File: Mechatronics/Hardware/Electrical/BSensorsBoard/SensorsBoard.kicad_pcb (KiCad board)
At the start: 2 copper layers, 49.8 x 13.7 mm, 10 parts, among them J1 Conn_01x01_Male, J2 Conn_01x01_Male, J3 Conn_01x01_Male, J4 Conn_01x01_Male, J5 Conn_01x01_Male, J6 Conn_01x01_Male, J7 Conn_01x01_Male, J8 Conn_01x01_Male, U1 ITR1802, U2 ITR1802

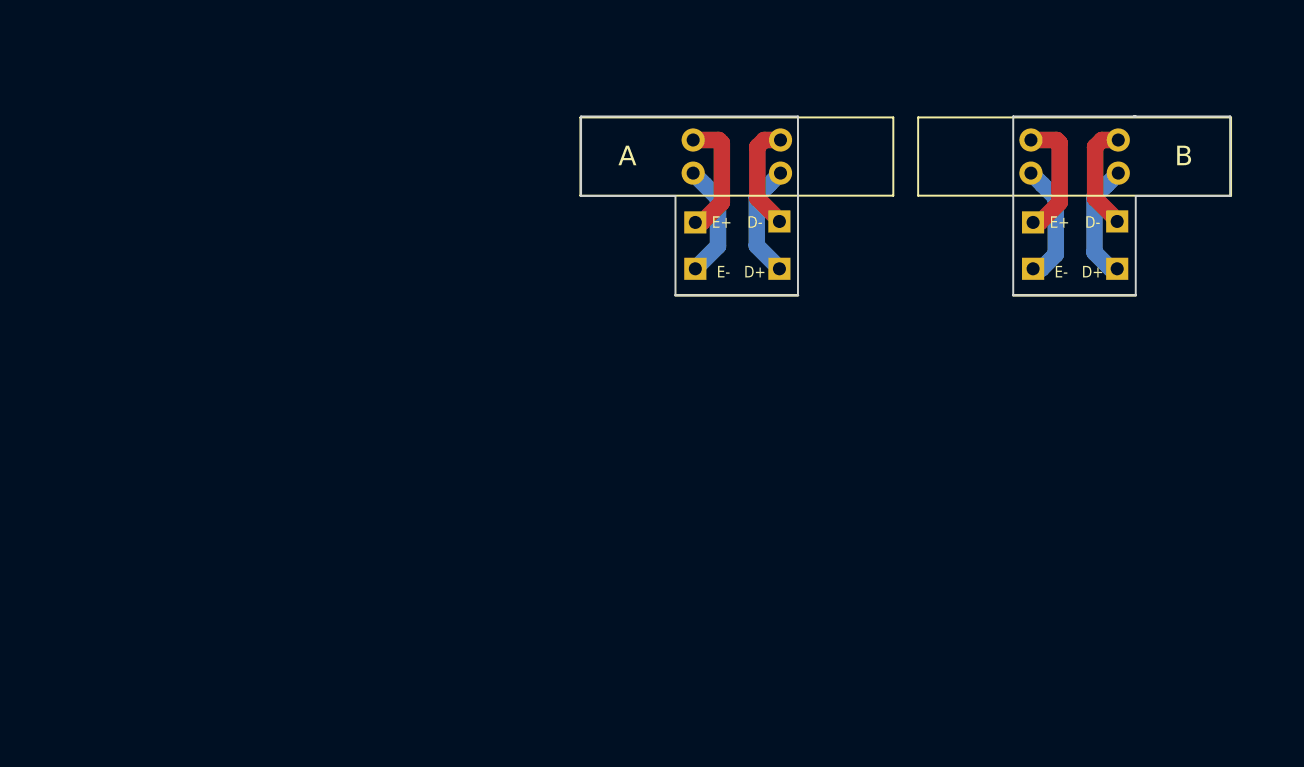
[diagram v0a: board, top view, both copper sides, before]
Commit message: Added changes
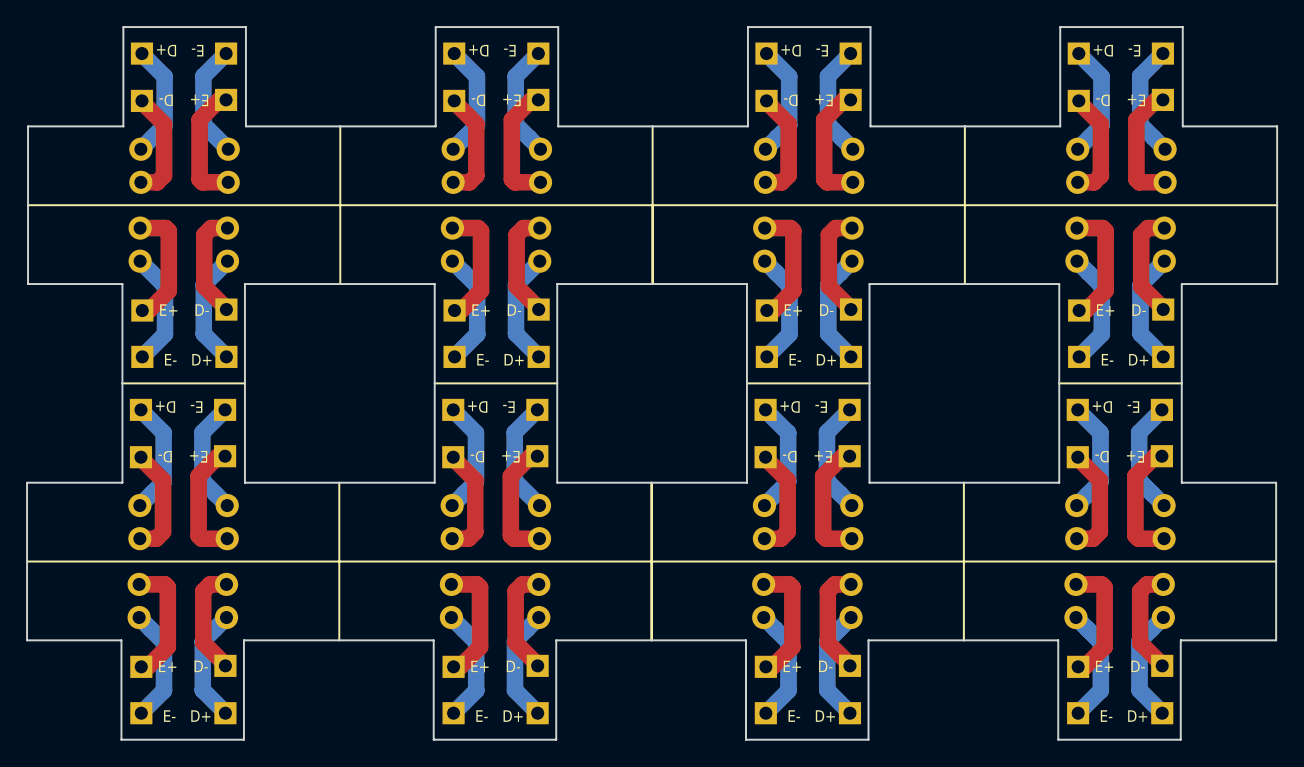
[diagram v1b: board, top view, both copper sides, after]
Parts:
- removed J5, J6, J7, J8: Conn_01x01_Male, Encoder:No3dmodelPinHeader_1x01_P2.54mm_Vertical
- removed U2: ITR1802, Encoder:itr8102
- added J1: Conn_01x01_Male, Encoder:No3dmodelPinHeader_1x01_P2.54mm_Vertical, F.Cu at (150.7, 120.2)
- added J1: Conn_01x01_Male, Encoder:No3dmodelPinHeader_1x01_P2.54mm_Vertical, F.Cu at (109.3, 76.7)
- added J1: Conn_01x01_Male, Encoder:No3dmodelPinHeader_1x01_P2.54mm_Vertical, F.Cu at (126.8, 92.9)
- added J1: Conn_01x01_Male, Encoder:No3dmodelPinHeader_1x01_P2.54mm_Vertical, F.Cu at (102.9, 92.9)
- added J1: Conn_01x01_Male, Encoder:No3dmodelPinHeader_1x01_P2.54mm_Vertical, F.Cu at (109.2, 104.0)
- added J1: Conn_01x01_Male, Encoder:No3dmodelPinHeader_1x01_P2.54mm_Vertical, F.Cu at (133.2, 104.0)
- added J1: Conn_01x01_Male, Encoder:No3dmodelPinHeader_1x01_P2.54mm_Vertical, F.Cu at (126.7, 120.2)
- added J1: Conn_01x01_Male, Encoder:No3dmodelPinHeader_1x01_P2.54mm_Vertical, F.Cu at (174.7, 120.2)
- added J1: Conn_01x01_Male, Encoder:No3dmodelPinHeader_1x01_P2.54mm_Vertical, F.Cu at (157.1, 104.0)
- added J1: Conn_01x01_Male, Encoder:No3dmodelPinHeader_1x01_P2.54mm_Vertical, F.Cu at (181.1, 104.0)
- added J1: Conn_01x01_Male, Encoder:No3dmodelPinHeader_1x01_P2.54mm_Vertical, F.Cu at (150.8, 92.9)
- added J1: Conn_01x01_Male, Encoder:No3dmodelPinHeader_1x01_P2.54mm_Vertical, F.Cu at (174.7, 92.9)
- added J1: Conn_01x01_Male, Encoder:No3dmodelPinHeader_1x01_P2.54mm_Vertical, F.Cu at (157.2, 76.7)
- added J1: Conn_01x01_Male, Encoder:No3dmodelPinHeader_1x01_P2.54mm_Vertical, F.Cu at (181.2, 76.7)
- added J1: Conn_01x01_Male, Encoder:No3dmodelPinHeader_1x01_P2.54mm_Vertical, F.Cu at (133.2, 76.7)
- added J2: Conn_01x01_Male, Encoder:No3dmodelPinHeader_1x01_P2.54mm_Vertical, F.Cu at (150.8, 96.4)
- added J2: Conn_01x01_Male, Encoder:No3dmodelPinHeader_1x01_P2.54mm_Vertical, F.Cu at (102.9, 96.4)
- added J2: Conn_01x01_Male, Encoder:No3dmodelPinHeader_1x01_P2.54mm_Vertical, F.Cu at (133.2, 73.2)
- added J2: Conn_01x01_Male, Encoder:No3dmodelPinHeader_1x01_P2.54mm_Vertical, F.Cu at (126.8, 96.4)
- added J2: Conn_01x01_Male, Encoder:No3dmodelPinHeader_1x01_P2.54mm_Vertical, F.Cu at (109.2, 100.5)
- added J2: Conn_01x01_Male, Encoder:No3dmodelPinHeader_1x01_P2.54mm_Vertical, F.Cu at (133.2, 100.5)
- added J2: Conn_01x01_Male, Encoder:No3dmodelPinHeader_1x01_P2.54mm_Vertical, F.Cu at (126.7, 123.7)
- added J2: Conn_01x01_Male, Encoder:No3dmodelPinHeader_1x01_P2.54mm_Vertical, F.Cu at (174.7, 123.7)
- added J2: Conn_01x01_Male, Encoder:No3dmodelPinHeader_1x01_P2.54mm_Vertical, F.Cu at (181.1, 100.5)
- added J2: Conn_01x01_Male, Encoder:No3dmodelPinHeader_1x01_P2.54mm_Vertical, F.Cu at (150.7, 123.7)
- added J2: Conn_01x01_Male, Encoder:No3dmodelPinHeader_1x01_P2.54mm_Vertical, F.Cu at (157.1, 100.5)
- added J2: Conn_01x01_Male, Encoder:No3dmodelPinHeader_1x01_P2.54mm_Vertical, F.Cu at (157.2, 73.2)
- added J2: Conn_01x01_Male, Encoder:No3dmodelPinHeader_1x01_P2.54mm_Vertical, F.Cu at (181.2, 73.2)
- added J2: Conn_01x01_Male, Encoder:No3dmodelPinHeader_1x01_P2.54mm_Vertical, F.Cu at (174.7, 96.4)
- added J2: Conn_01x01_Male, Encoder:No3dmodelPinHeader_1x01_P2.54mm_Vertical, F.Cu at (109.3, 73.2)
- added J3: Conn_01x01_Male, Encoder:No3dmodelPinHeader_1x01_P2.54mm_Vertical, F.Cu at (150.7, 76.8)
- added J3: Conn_01x01_Male, Encoder:No3dmodelPinHeader_1x01_P2.54mm_Vertical, F.Cu at (109.3, 92.8)
- added J3: Conn_01x01_Male, Encoder:No3dmodelPinHeader_1x01_P2.54mm_Vertical, F.Cu at (102.8, 76.8)
- added J3: Conn_01x01_Male, Encoder:No3dmodelPinHeader_1x01_P2.54mm_Vertical, F.Cu at (133.3, 92.8)
- added J3: Conn_01x01_Male, Encoder:No3dmodelPinHeader_1x01_P2.54mm_Vertical, F.Cu at (126.7, 104.1)
- added J3: Conn_01x01_Male, Encoder:No3dmodelPinHeader_1x01_P2.54mm_Vertical, F.Cu at (102.8, 104.1)
- added J3: Conn_01x01_Male, Encoder:No3dmodelPinHeader_1x01_P2.54mm_Vertical, F.Cu at (133.2, 120.1)
- added J3: Conn_01x01_Male, Encoder:No3dmodelPinHeader_1x01_P2.54mm_Vertical, F.Cu at (157.1, 120.1)
- added J3: Conn_01x01_Male, Encoder:No3dmodelPinHeader_1x01_P2.54mm_Vertical, F.Cu at (181.2, 92.8)
- added J3: Conn_01x01_Male, Encoder:No3dmodelPinHeader_1x01_P2.54mm_Vertical, F.Cu at (174.6, 104.1)
- added J3: Conn_01x01_Male, Encoder:No3dmodelPinHeader_1x01_P2.54mm_Vertical, F.Cu at (181.1, 120.1)
- added J3: Conn_01x01_Male, Encoder:No3dmodelPinHeader_1x01_P2.54mm_Vertical, F.Cu at (150.7, 104.1)
- added J3: Conn_01x01_Male, Encoder:No3dmodelPinHeader_1x01_P2.54mm_Vertical, F.Cu at (157.2, 92.8)
- added J3: Conn_01x01_Male, Encoder:No3dmodelPinHeader_1x01_P2.54mm_Vertical, F.Cu at (174.7, 76.8)
- added J3: Conn_01x01_Male, Encoder:No3dmodelPinHeader_1x01_P2.54mm_Vertical, F.Cu at (126.8, 76.8)
- added J4: Conn_01x01_Male, Encoder:No3dmodelPinHeader_1x01_P2.54mm_Vertical, F.Cu at (150.7, 73.2)
- added J4: Conn_01x01_Male, Encoder:No3dmodelPinHeader_1x01_P2.54mm_Vertical, F.Cu at (126.8, 73.2)
- added J4: Conn_01x01_Male, Encoder:No3dmodelPinHeader_1x01_P2.54mm_Vertical, F.Cu at (102.8, 73.2)
- added J4: Conn_01x01_Male, Encoder:No3dmodelPinHeader_1x01_P2.54mm_Vertical, F.Cu at (133.3, 96.4)
- added J4: Conn_01x01_Male, Encoder:No3dmodelPinHeader_1x01_P2.54mm_Vertical, F.Cu at (126.7, 100.5)
- added J4: Conn_01x01_Male, Encoder:No3dmodelPinHeader_1x01_P2.54mm_Vertical, F.Cu at (102.8, 100.5)
- added J4: Conn_01x01_Male, Encoder:No3dmodelPinHeader_1x01_P2.54mm_Vertical, F.Cu at (133.2, 123.7)
- added J4: Conn_01x01_Male, Encoder:No3dmodelPinHeader_1x01_P2.54mm_Vertical, F.Cu at (174.6, 100.5)
- added J4: Conn_01x01_Male, Encoder:No3dmodelPinHeader_1x01_P2.54mm_Vertical, F.Cu at (157.1, 123.7)
- added J4: Conn_01x01_Male, Encoder:No3dmodelPinHeader_1x01_P2.54mm_Vertical, F.Cu at (181.1, 123.7)
- added J4: Conn_01x01_Male, Encoder:No3dmodelPinHeader_1x01_P2.54mm_Vertical, F.Cu at (174.7, 73.2)
- added J4: Conn_01x01_Male, Encoder:No3dmodelPinHeader_1x01_P2.54mm_Vertical, F.Cu at (181.2, 96.4)
- added J4: Conn_01x01_Male, Encoder:No3dmodelPinHeader_1x01_P2.54mm_Vertical, F.Cu at (157.2, 96.4)
- added J4: Conn_01x01_Male, Encoder:No3dmodelPinHeader_1x01_P2.54mm_Vertical, F.Cu at (150.7, 100.5)
- added J4: Conn_01x01_Male, Encoder:No3dmodelPinHeader_1x01_P2.54mm_Vertical, F.Cu at (109.3, 96.4)
- added U1: ITR1802, Encoder:itr8102, F.Cu at (154.0, 87.8)
- added U1: ITR1802, Encoder:itr8102, F.Cu at (130.1, 81.8)
- added U1: ITR1802, Encoder:itr8102, F.Cu at (106.1, 81.8)
- added U1: ITR1802, Encoder:itr8102, F.Cu at (130.0, 87.8)
- added U1: ITR1802, Encoder:itr8102, F.Cu at (130.0, 109.1)
- added U1: ITR1802, Encoder:itr8102, F.Cu at (106.0, 109.1)
- added U1: ITR1802, Encoder:itr8102, F.Cu at (129.9, 115.1)
- added U1: ITR1802, Encoder:itr8102, F.Cu at (154.0, 81.8)
- added U1: ITR1802, Encoder:itr8102, F.Cu at (178.0, 81.8)
- added U1: ITR1802, Encoder:itr8102, F.Cu at (177.9, 87.8)
- added U1: ITR1802, Encoder:itr8102, F.Cu at (177.9, 109.1)
- added U1: ITR1802, Encoder:itr8102, F.Cu at (153.9, 115.1)
- added U1: ITR1802, Encoder:itr8102, F.Cu at (177.8, 115.1)
- added U1: ITR1802, Encoder:itr8102, F.Cu at (153.9, 109.1)
- added U1: ITR1802, Encoder:itr8102, F.Cu at (106.1, 87.8)
- moved J1 54.5 mm to (102.8, 120.2)
- moved J3 54.5 mm to (109.2, 120.1)
- moved U1 54.5 mm to (106.0, 115.1)
- moved J2 54.5 mm to (102.8, 123.7)
- moved J4 54.5 mm to (109.2, 123.7)
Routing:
- net (no net): track 0.00 -> 534.2 mm
- net Net-(J5-Pad1): track 9.53 -> 0.00 mm
- net Net-(J6-Pad1): track 9.22 -> 0.00 mm
- net Net-(J8-Pad1): track 9.10 -> 0.00 mm
- net Net-(J7-Pad1): track 8.42 -> 0.00 mm
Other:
- board size 49.8 x 13.7 mm -> 95.9 x 54.7 mm
- board text removed: "A"
- board text removed: "B"
